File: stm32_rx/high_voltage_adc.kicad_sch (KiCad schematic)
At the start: 15 parts, among them U11 AMC1351DWV, U18 ISO7760DW, U4 AMC1351DWV, U9 ACS709xLFTR-20BB

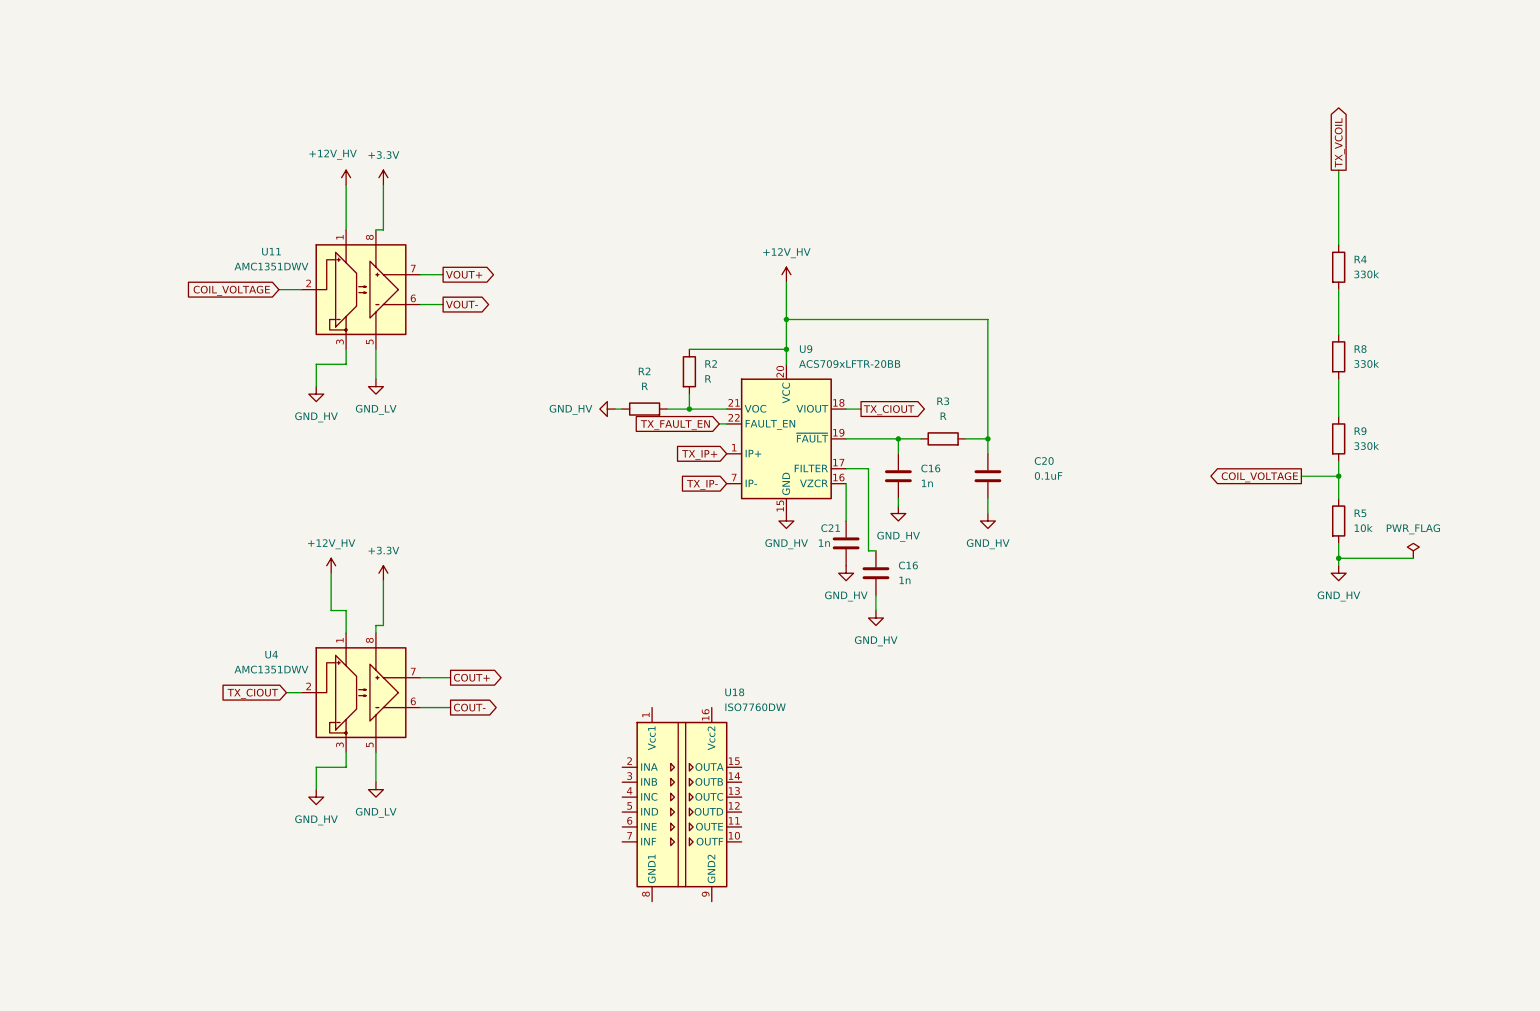
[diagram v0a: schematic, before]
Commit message: I can't find the right module
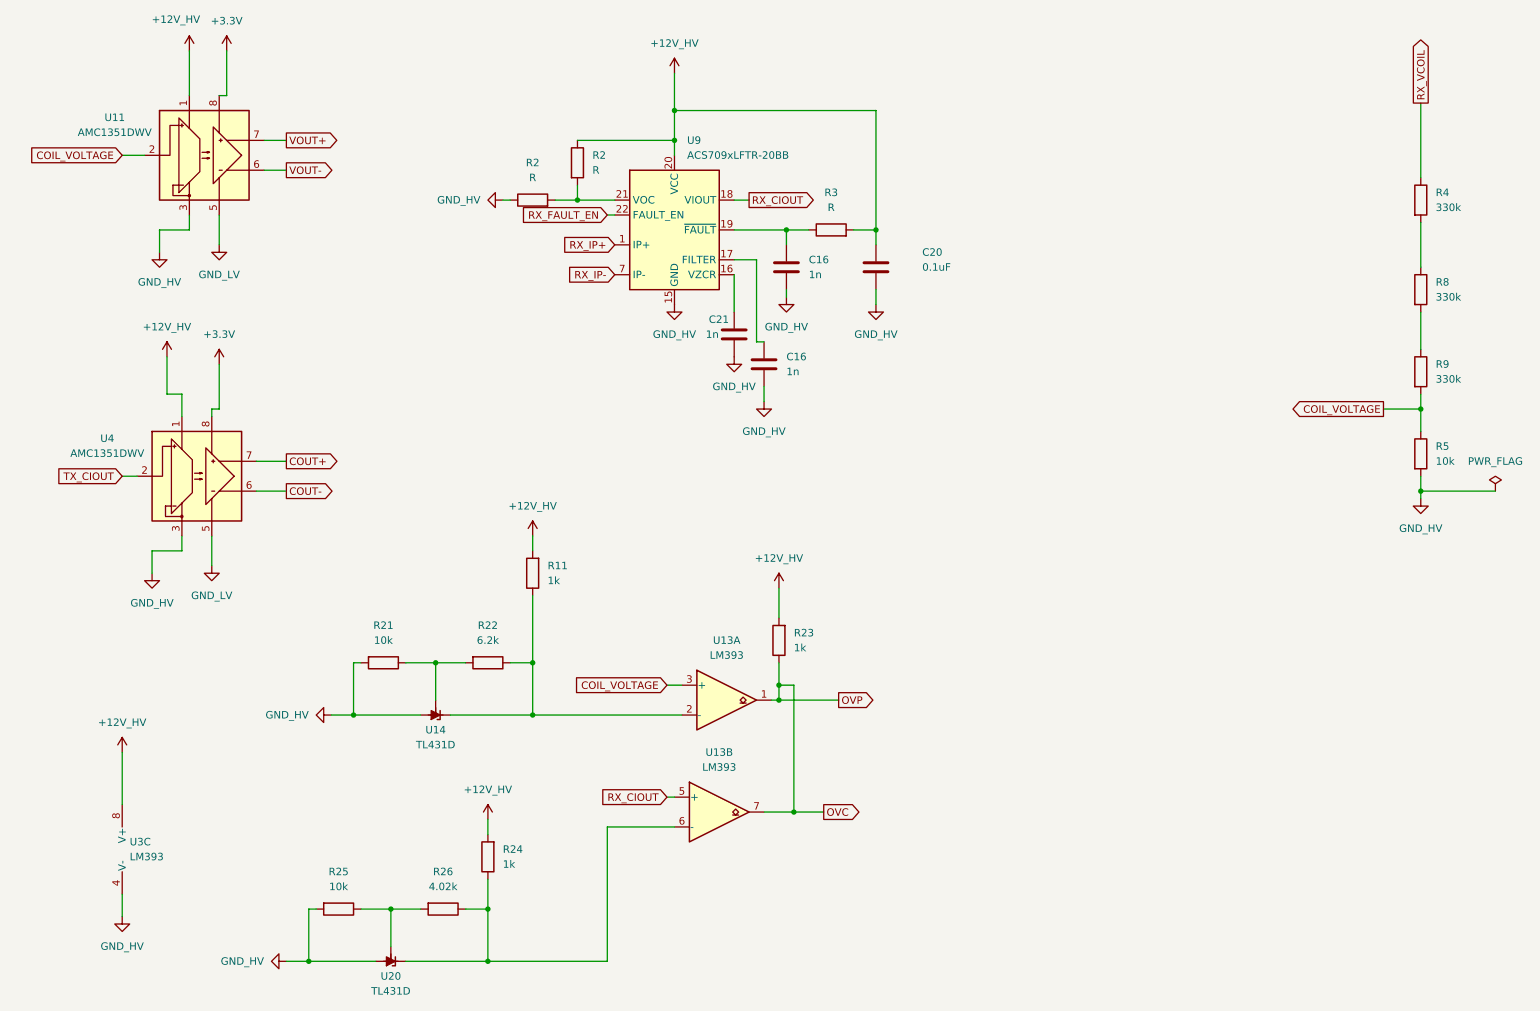
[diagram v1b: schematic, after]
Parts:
- removed U18: ISO7760DW, Package_SO:SOIC-16W_7.5x10.3mm_P1.27mm, symbol Isolator:ISO7760DW
- added R11: 1k, Resistor_SMD:R_0402_1005Metric, symbol Device:R
- added R21, R25: 10k, Resistor_SMD:R_1206_3216Metric, symbol Device:R
- added R22: 6.2k, Resistor_SMD:R_1206_3216Metric, symbol Device:R
- added R23, R24: 1k, Resistor_SMD:R_1206_3216Metric, symbol Device:R
- added R26: 4.02k, Resistor_SMD:R_1206_3216Metric, symbol Device:R
- added U13, U3: LM393, symbol Comparator:LM393
- added U14, U20: TL431D, Package_SO:SOIC-8_3.9x4.9mm_P1.27mm, symbol Reference_Voltage:TL431D
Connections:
- net +12V_HV: now also R11.2, R23.2, R24.2, U3.8 (V+)
- net COIL_VOLTAGE: now also U13.3 (+)
- net GND_HV: now also R21.2, R25.2, U14.2 (A), U14.3 (A), U14.6 (A), U14.7 (A), U20.2 (A), U20.3 (A), U20.6 (A), U20.7 (A), U3.4 (V-)
- net TX_CIOUT: no longer U9.18 (VIOUT)
- net TX_FAULT_EN renamed RX_FAULT_EN
- net TX_IP+ renamed RX_IP+
- net TX_IP- renamed RX_IP-
- net TX_VCOIL renamed RX_VCOIL
- new net: R21.1, R22.2, U14.8 (REF)
- new net: R24.1, R26.1, U13.6 (-), U20.1 (K)
- new net: R25.1, R26.2, U20.8 (REF)
- new net: R11.1, R22.1, U13.2 (-), U14.1 (K)
- new net OVC: R23.1, U13.1, U13.7
- new net RX_CIOUT: U13.5 (+), U9.18 (VIOUT)
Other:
- moved on the sheet: C16, C20, C21, R2, R3, R4, R5, R8, R9, U11, U4, U9
